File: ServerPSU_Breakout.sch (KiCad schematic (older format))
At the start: 0 parts

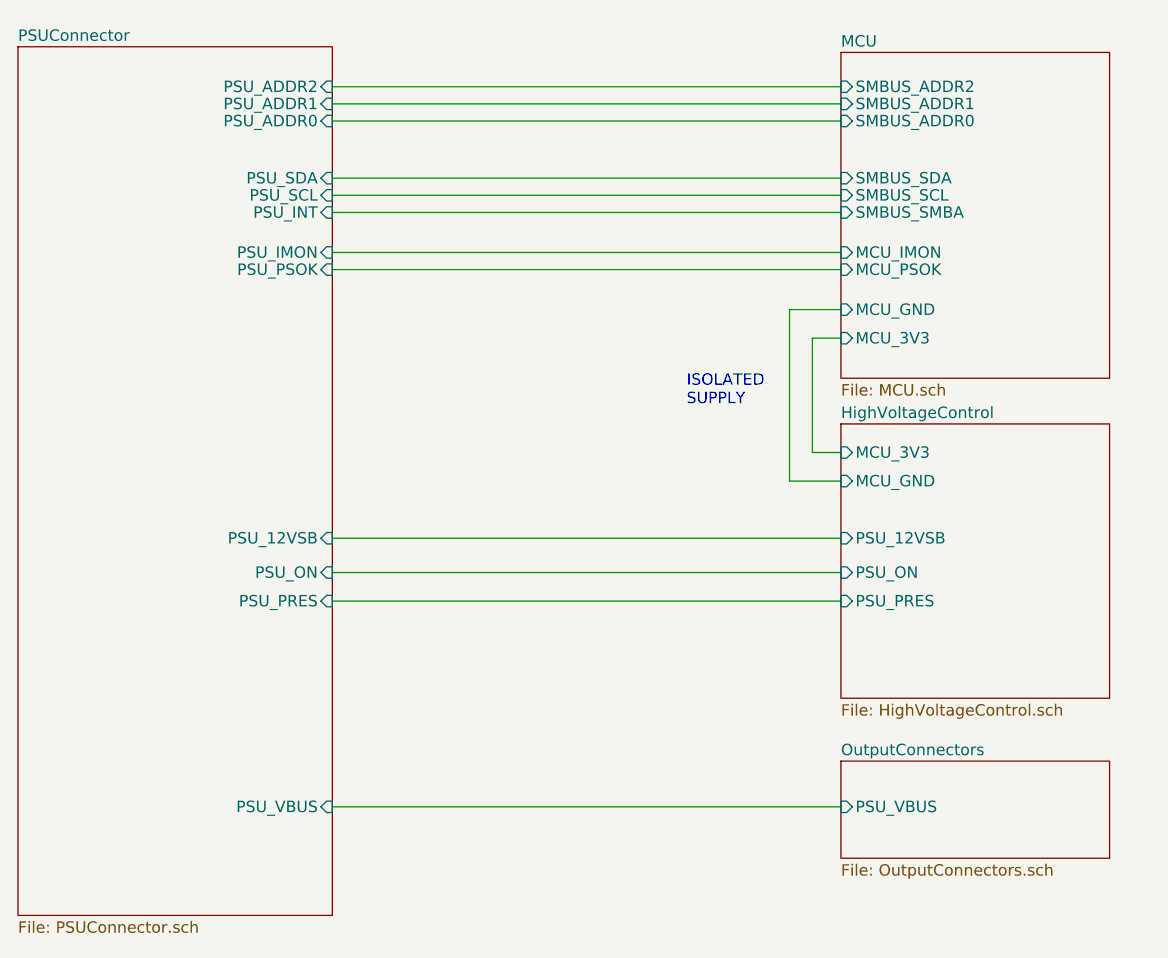
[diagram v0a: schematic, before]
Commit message: layout draft
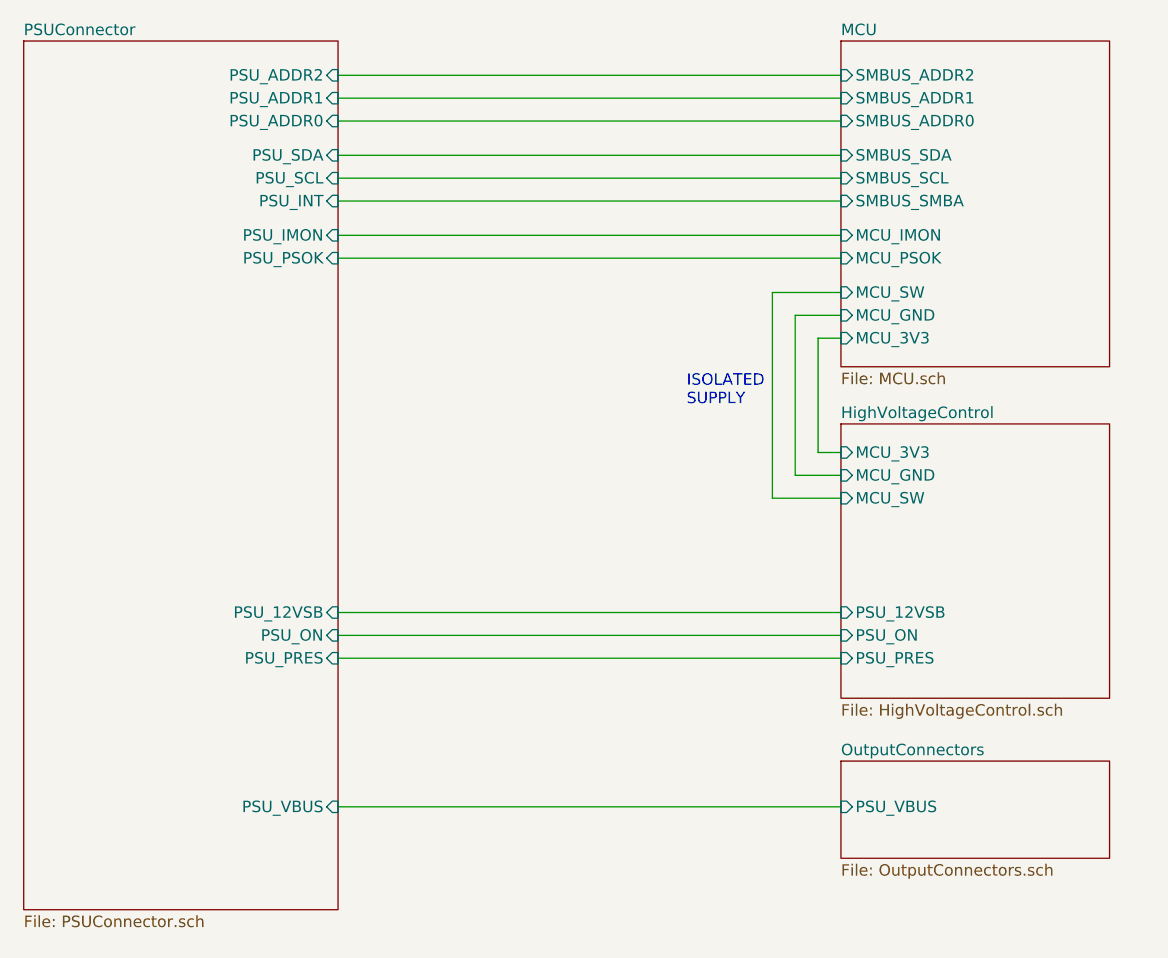
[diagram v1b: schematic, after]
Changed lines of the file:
@@
 F0 "HighVoltageControl" 50
 F1 "HighVoltageControl.sch" 50
-F2 "PSU_12VSB" I L 5250 5125 50
-F3 "MCU_GND" I L 5250 4875 50
+F2 "PSU_12VSB" I L 5250 5450 50
+F3 "MCU_GND" I L 5250 4850 50
 F4 "MCU_3V3" I L 5250 4750 50
-F5 "PSU_ON" I L 5250 5275 50
-F6 "PSU_PRES" I L 5250 5400 50
+F5 "PSU_ON" I L 5250 5550 50
+F6 "PSU_PRES" I L 5250 5650 50
+F7 "MCU_SW" I L 5250 4950 50
 $EndSheet
+Wire Wire Line
+	5250 5650 3050 5650
+Wire Wire Line
+	3050 5550 5250 5550
+Wire Wire Line
+	3050 5450 5250 5450
+Wire Wire Line
+	5250 6300 3050 6300
+Text Notes 4575 4550 0    50   ~ 0
+ISOLATED\nSUPPLY
+Wire Wire Line
+	5250 3300 3050 3300
+Wire Wire Line
+	5250 3200 3050 3200
+Wire Wire Line
+	5250 3100 3050 3100
 $Sheet
-S 5250 3000 1175 1425
+S 5250 2950 1175 1425
 U 5F02F4E9
 F0 "MCU" 50
 F1 "MCU.sch" 50
-F2 "MCU_GND" I L 5250 4125 50
+F2 "MCU_GND" I L 5250 4150 50
 F3 "MCU_3V3" I L 5250 4250 50
-F4 "MCU_PSOK" I L 5250 3950 50
-F5 "SMBUS_SDA" I L 5250 3550 50
-F6 "SMBUS_SCL" I L 5250 3625 50
-F7 "SMBUS_SMBA" I L 5250 3700 50
+F4 "MCU_PSOK" I L 5250 3900 50
+F5 "SMBUS_SDA" I L 5250 3450 50
+F6 "SMBUS_SCL" I L 5250 3550 50
+F7 "SMBUS_SMBA" I L 5250 3650 50
 F8 "SMBUS_ADDR0" I L 5250 3300 50
-F9 "SMBUS_ADDR1" I L 5250 3225 50
-F10 "SMBUS_ADDR2" I L 5250 3150 50
-F11 "MCU_IMON" I L 5250 3875 50
+F9 "SMBUS_ADDR1" I L 5250 3200 50
+F10 "SMBUS_ADDR2" I L 5250 3100 50
+F11 "MCU_IMON" I L 5250 3800 50
+F12 "MCU_SW" I L 5250 4050 50
 $EndSheet
-Wire Wire Line
-	5250 5400 3025 5400
-Wire Wire Line
-	3025 5275 5250 5275
-Wire Wire Line
-	3025 5125 5250 5125
 $Sheet
-S 1650 2975 1375 3800
+S 1675 2950 1375 3800
 U 5EFF0F4B
 F0 "PSUConnector" 50
 F1 "PSUConnector.sch" 50
-F2 "PSU_VBUS" I R 3025 6300 50
-F3 "PSU_ADDR2" I R 3025 3150 50
-F4 "PSU_ADDR1" I R 3025 3225 50
-F5 "PSU_ADDR0" I R 3025 3300 50
-F6 "PSU_12VSB" I R 3025 5125 50
-F7 "PSU_PSOK" I R 3025 3950 50
-F8 "PSU_SDA" I R 3025 3550 50
-F9 "PSU_SCL" I R 3025 3625 50
-F10 "PSU_ON" I R 3025 5275 50
-F11 "PSU_PRES" I R 3025 5400 50
-F12 "PSU_IMON" I R 3025 3875 50
-F13 "PSU_INT" I R 3025 3700 50
+F2 "PSU_VBUS" I R 3050 6300 50
+F3 "PSU_ADDR2" I R 3050 3100 50
+F4 "PSU_ADDR1" I R 3050 3200 50
+F5 "PSU_ADDR0" I R 3050 3300 50
+F6 "PSU_12VSB" I R 3050 5450 50
+F7 "PSU_PSOK" I R 3050 3900 50
+F8 "PSU_SDA" I R 3050 3450 50
+F9 "PSU_SCL" I R 3050 3550 50
+F10 "PSU_ON" I R 3050 5550 50
+F11 "PSU_PRES" I R 3050 5650 50
+F12 "PSU_IMON" I R 3050 3800 50
+F13 "PSU_INT" I R 3050 3650 50
 $EndSheet
 Wire Wire Line
-	5250 6300 3025 6300
+	3050 3450 5250 3450
 Wire Wire Line
-	5250 4750 5125 4750
+	5250 3550 3050 3550
 Wire Wire Line
-	5125 4250 5250 4250
+	5250 3650 3050 3650
 Wire Wire Line
-	5025 4125 5025 4875
+	5250 3800 3050 3800
 Wire Wire Line
-	5025 4875 5250 4875
+	5250 3900 3050 3900
 Wire Wire Line
-	5025 4125 5250 4125
+	5250 4850 5050 4850
 Wire Wire Line
-	5250 3950 3025 3950
+	5050 4850 5050 4150
 Wire Wire Line
-	5250 3875 3025 3875
+	5050 4150 5250 4150
 Wire Wire Line
-	5125 4750 5125 4250
+	5250 4950 4950 4950
 Wire Wire Line
-	5250 3550 3025 3550
+	4950 4950 4950 4050
 Wire Wire Line
-	3025 3625 5250 3625
+	4950 4050 5250 4050
 Wire Wire Line
-	3025 3700 5250 3700
+	5250 4250 5150 4250
 Wire Wire Line
-	5250 3150 3025 3150
+	5150 4250 5150 4750
 Wire Wire Line
-	3025 3225 5250 3225
-Wire Wire Line
-	5250 3300 3025 3300
-Text Notes 4575 4550 0    50   ~ 0
-ISOLATED\nSUPPLY
+	5150 4750 5250 4750
 $EndSCHEMATC
